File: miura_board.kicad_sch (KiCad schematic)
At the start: 26 parts, among them J1 Conn_01x02_Female, J2 Screw_Terminal_01x02, J3 Screw_Terminal_01x02, SW1 SW_Push, U1 ATmega32U4-A, U2 NRF24L01, U3 DRV8833PW, U4 DRV8833PW, Y1 16MHz, Y2 16MHz

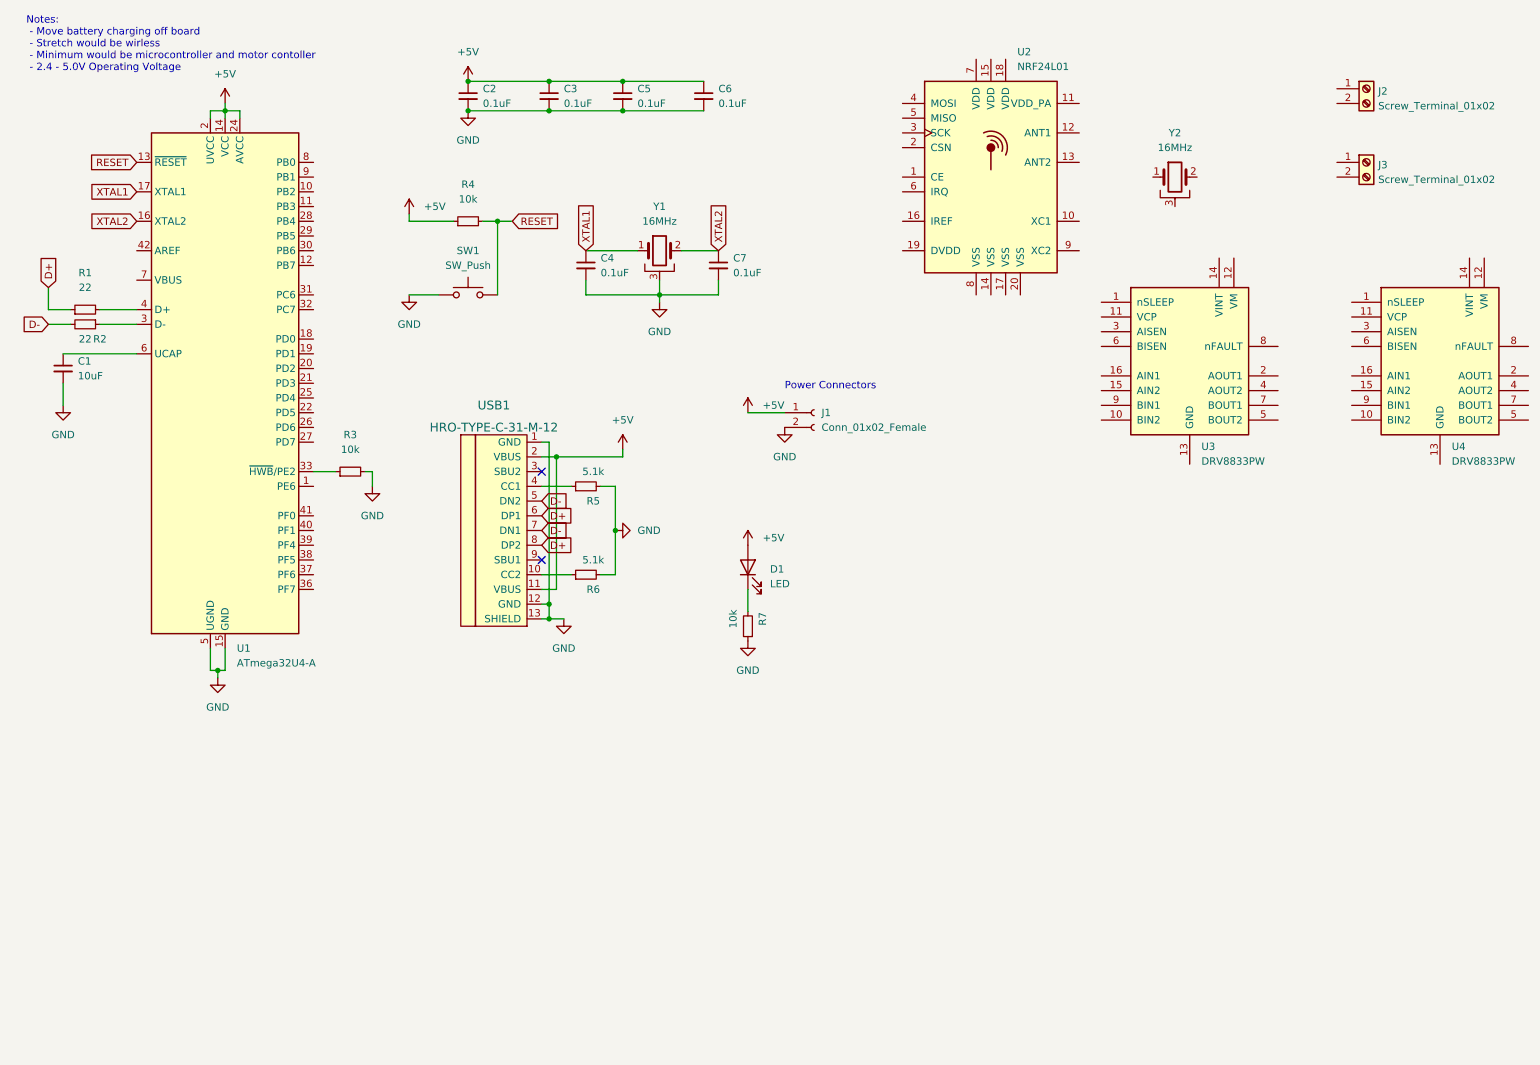
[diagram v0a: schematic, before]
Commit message: Square
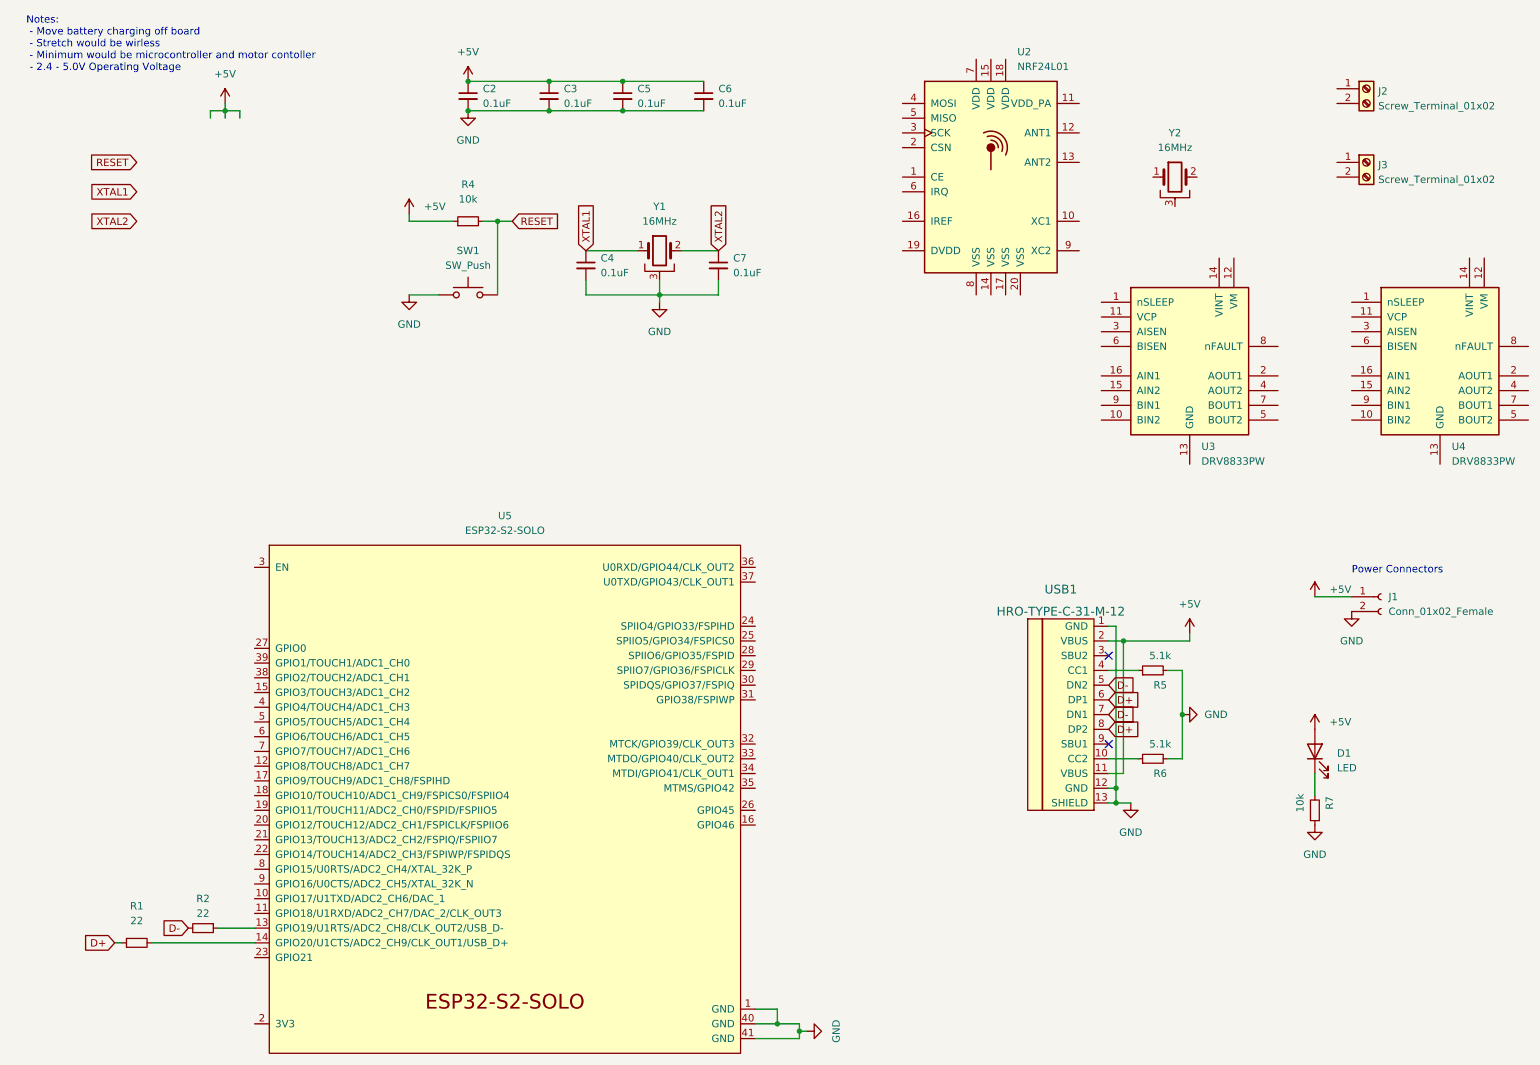
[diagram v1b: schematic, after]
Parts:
- removed C1: 10uF, Capacitor_SMD:C_0603_1608Metric, symbol Device:C_Small
- removed R3: 10k, Resistor_SMD:R_0603_1608Metric_Pad0.98x0.95mm_HandSolder, symbol Device:R_Small
- removed U1: ATmega32U4-A, Package_QFP:TQFP-44_10x10mm_P0.8mm, symbol MCU_Microchip_ATmega:ATmega32U4-A
- added U5: ESP32-S2-SOLO, Espressif:ESP32-S2-SOLO, symbol Espressif:ESP32-S2-SOLO
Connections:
- net GND: now also U5.1 (GND), U5.40 (GND), U5.41 (GND)
- net at R2.1: now also U5.13 (GPIO19/U1RTS/ADC2_CH8/CLK_OUT2/USB_D-)
- net at R1.2: now also U5.14 (GPIO20/U1CTS/ADC2_CH9/CLK_OUT1/USB_D+)
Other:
- moved on the sheet: D1, J1, R1, R2, R5, R6, R7, USB1
